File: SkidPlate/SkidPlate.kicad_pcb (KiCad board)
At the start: 4 copper layers, 100.8 x 26 mm, 27 parts, among them J1 Conn_02x09_Counter_Clockwise, J6 STEMMA_QT, J7 STEMMA_QT, U1 AMS1117-3.3, U2 LSM6DSOX

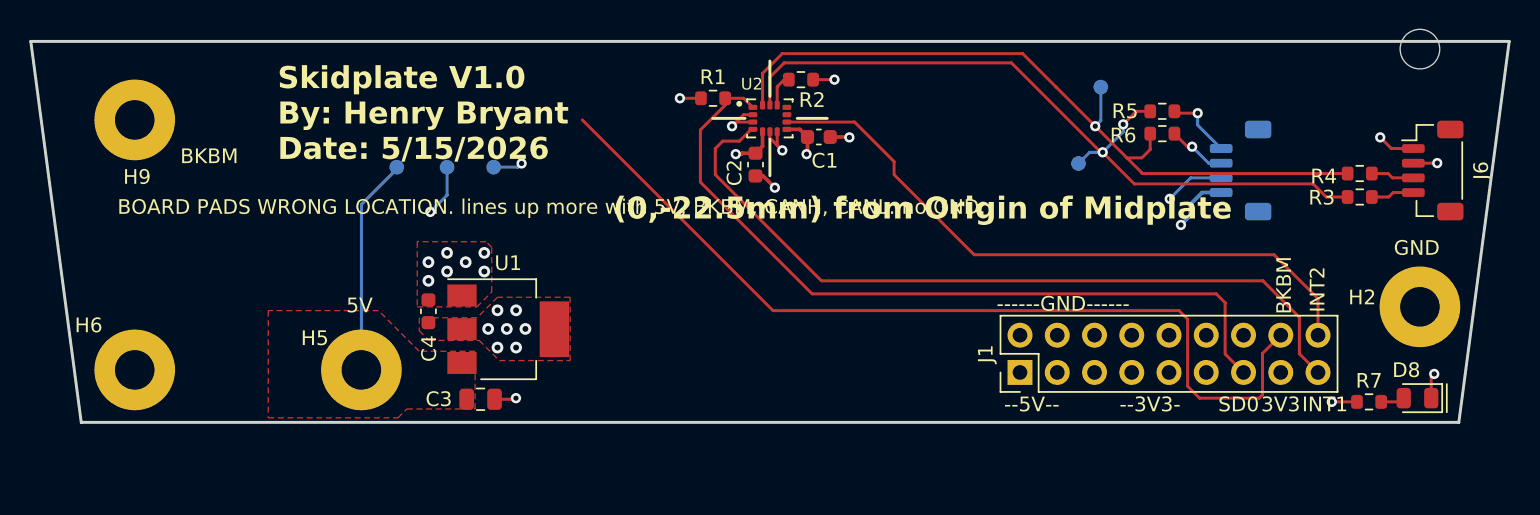
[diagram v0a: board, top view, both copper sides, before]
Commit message: skidplate done
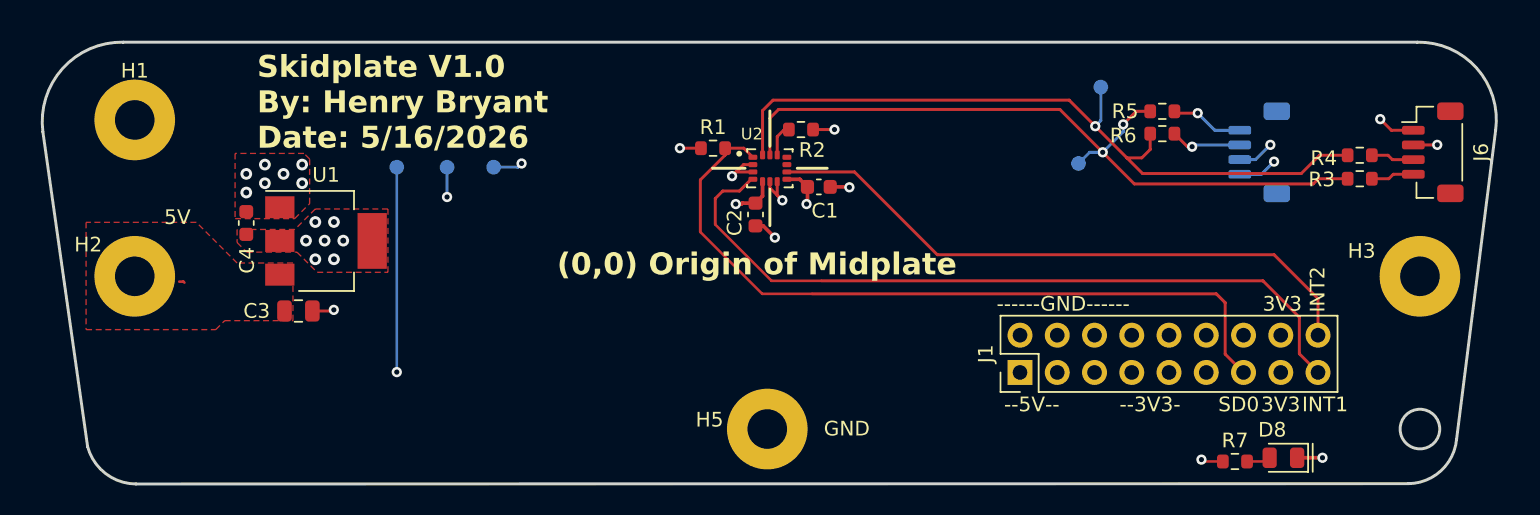
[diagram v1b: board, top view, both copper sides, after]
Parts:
- removed H6: EXTRA, bots:MountingHole_2.7mm_M2.5_DIN965_Pad
- removed H9: BKBM, bots:MountingHole_2.7mm_M2.5_DIN965_Pad
- removed REF**: MountingHole_No_copper_M2.5, bots:MountingHole_No_copper_M2.5
- added H1: RPI, bots:MountingHole_2.7mm_M2.5_DIN965_Pad, F.Cu at (107.7, 107.6)
- added H3: CANH, bots:MountingHole_2.7mm_M2.5_DIN965_Pad, F.Cu at (195.4, 118.3)
- moved H5 45.3 mm to (150.9, 128.7)
- moved H2 16.7 mm to (107.7, 118.3)
- moved C4 13.8 mm to (115.3, 114.7)
- moved C3 13.8 mm to (118.9, 120.7)
- moved U1 13.8 mm to (120.8, 115.9)
- moved R7 10.0 mm to (182.8, 130.9)
- moved D8 10.0 mm to (186.1, 130.7)
- moved C1 3.40 mm to (154.4, 112.2)
- moved C2 3.40 mm to (150.1, 114.1)
- moved R1 3.40 mm to (147.2, 109.6)
- moved R2 3.40 mm to (153.2, 108.3)
- moved U2 3.40 mm to (151.0, 110.9)
- moved J7 1.78 mm to (184.4, 109.9)
- moved R3 1.24 mm to (191.3, 111.7)
- moved R4 1.24 mm to (191.3, 110.1)
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- renumbered H5 to H2, H2 to H5
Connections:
- J1 pad 11: /BKBM -> +3V3
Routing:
- net /BKBM: track 61.6 -> 0.00 mm
- net GND: track 22.7 -> 19.8 mm
- net /INT2: track 44.2 -> 42.3 mm
- net +3V3: track 18.2 -> 16.4 mm
- net /INT1: track 53.0 -> 51.6 mm
- net /SD0: track 53.0 -> 51.6 mm
- net /IMU_SCL: track 52.1 -> 51.2 mm
- net Net-(J7-Pin_3): track 4.02 -> 4.87 mm
- net +5V: track 15.2 -> 14.5 mm, vias 0 -> 1
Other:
- board size 100.8 x 26 mm -> 99.1 x 30.1 mm
- board text added: "Skidplate V1.0 By: Henry Bryant Date: 5/16/2026"
- board text removed: "(0,-22.5mm) from Origin of Midplate"
- board text removed: "BKBM"
- board text removed: "BOARD PADS WRONG LOCATION. lines up more with 5V, BKBM, CANH, CANL. no GND."
- board text removed: "Skidplate V1.0 By: Henry Bryant Date: 5/15/2026"
